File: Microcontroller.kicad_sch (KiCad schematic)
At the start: 31 parts, among them SW1 KMR221GLFS, U4 STM32F446RET6, U7 W25Q128JVSIQ, Y1 16MHz

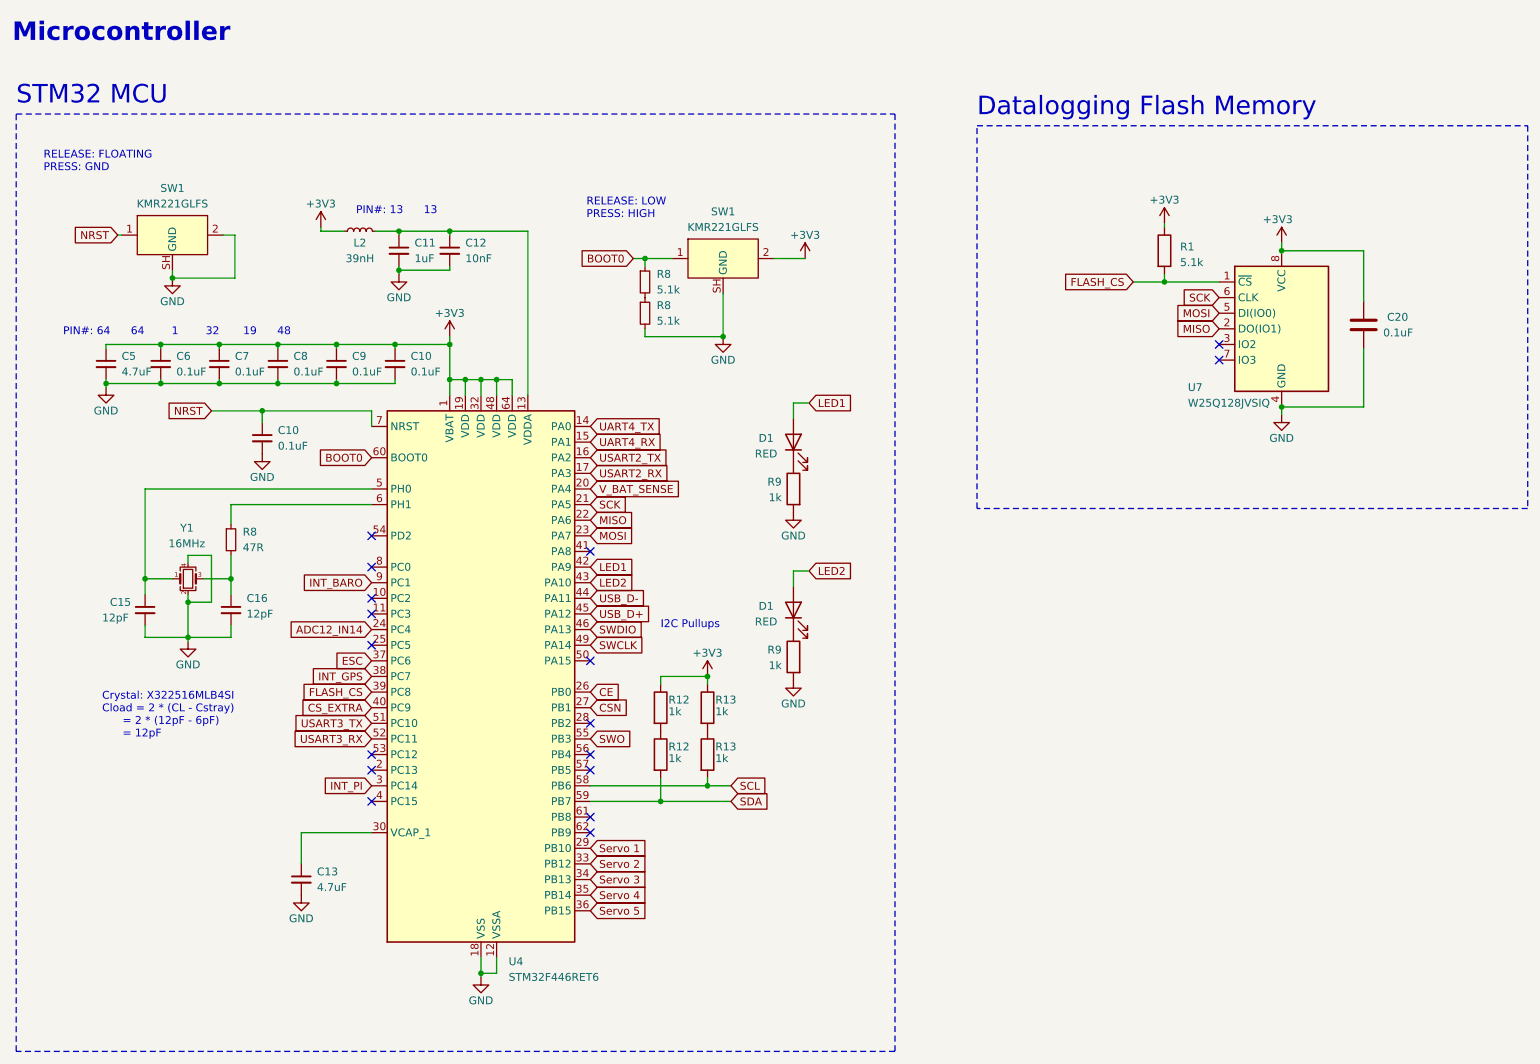
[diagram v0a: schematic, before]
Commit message: Add files via upload
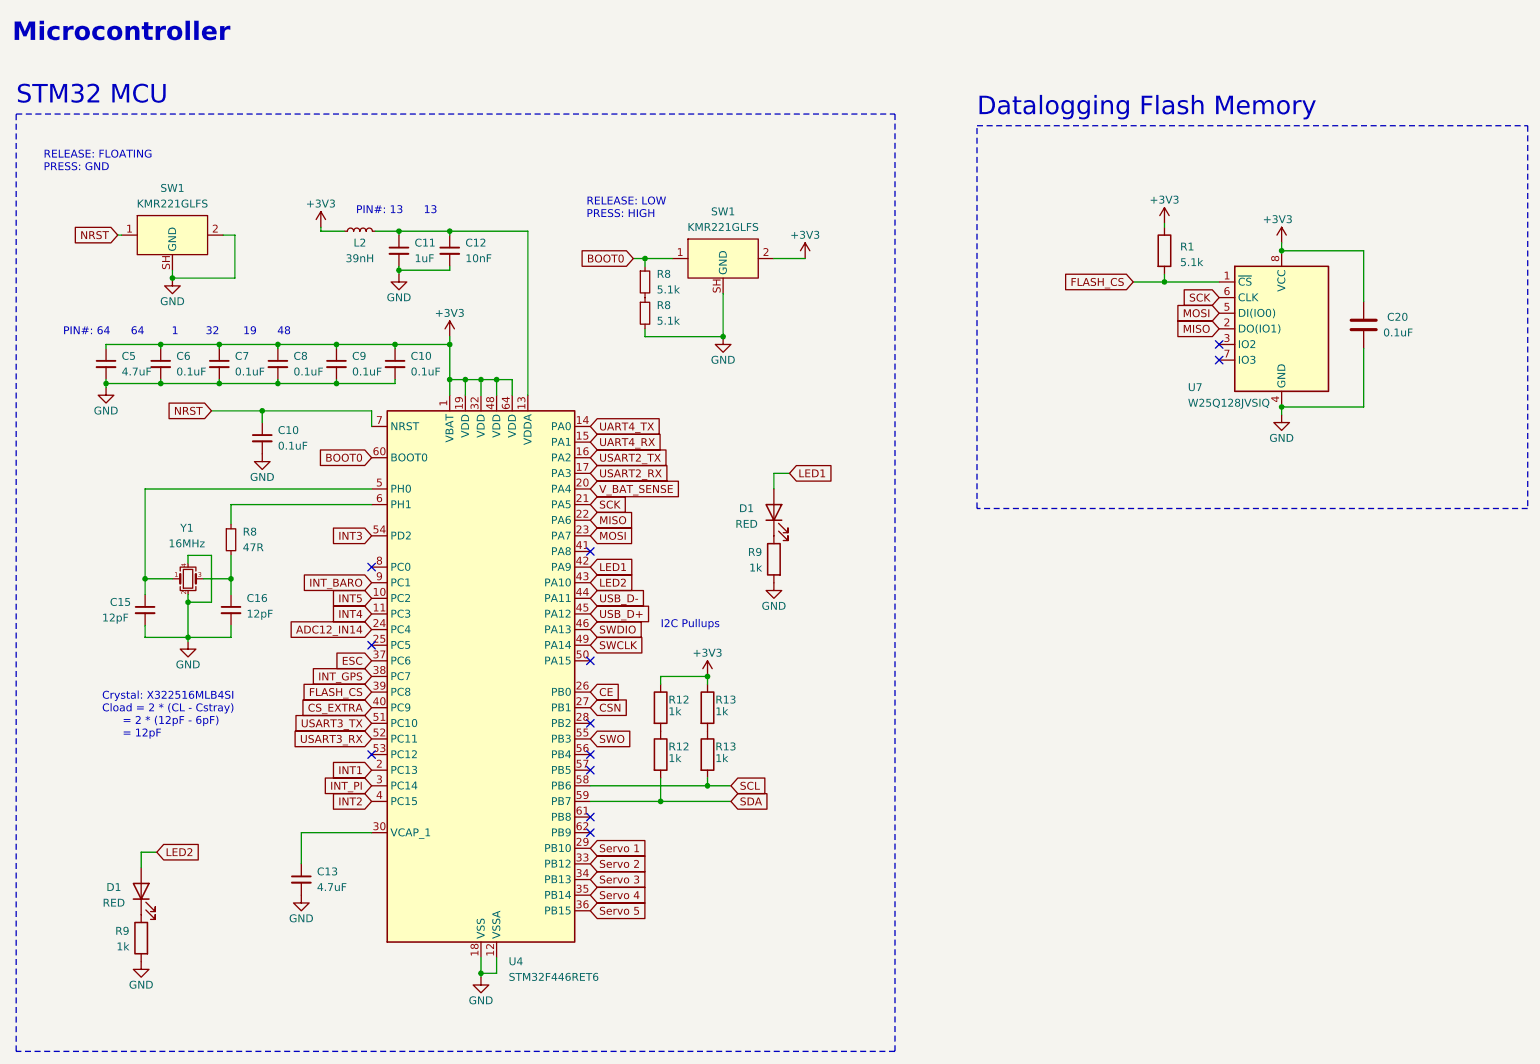
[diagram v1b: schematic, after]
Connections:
- net INT5: now reaches U4.10 (PC2)
- net INT4: now reaches U4.11 (PC3)
- net INT1: now reaches U4.2 (PC13)
- net INT2: now reaches U4.4 (PC15)
- net INT3: now reaches U4.54 (PD2)
- no-connect marks 17 -> 12
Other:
- moved on the sheet: D1, R9

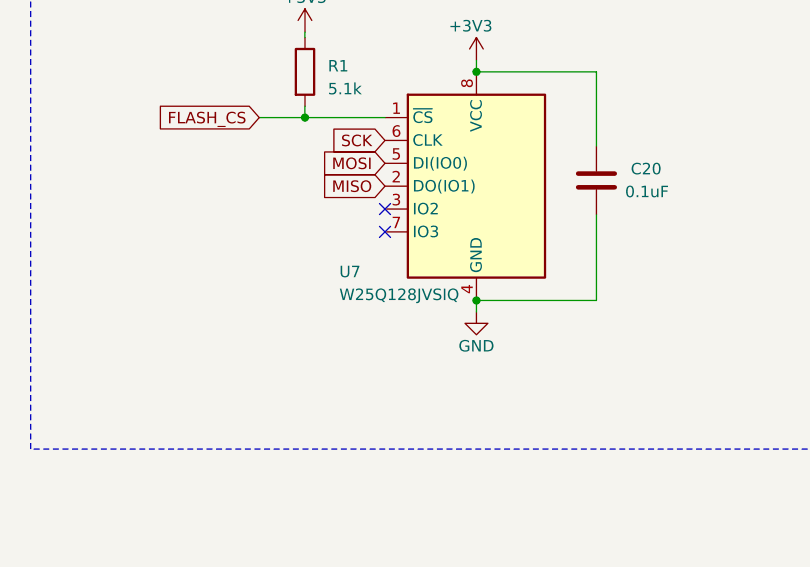
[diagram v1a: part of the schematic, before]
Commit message: Add files via upload
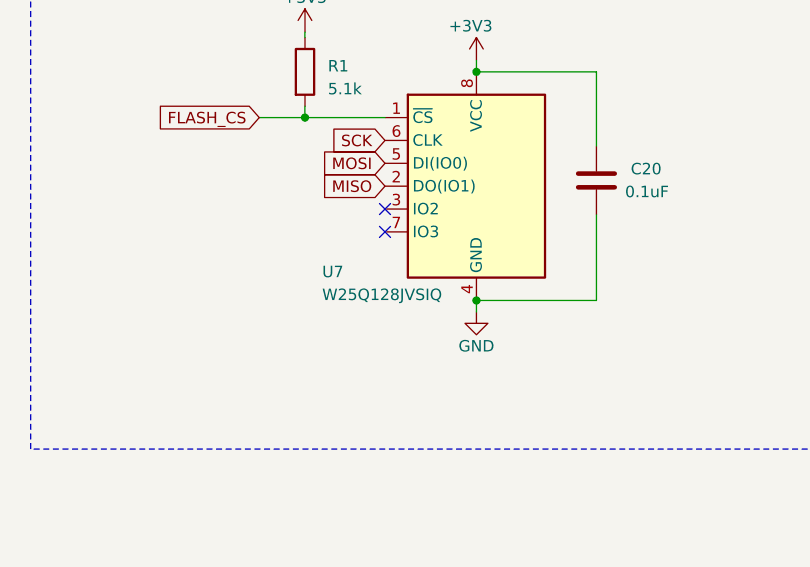
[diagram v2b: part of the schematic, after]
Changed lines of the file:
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@@
   (symbol (lib_id "Memory_Flash:W25Q128JVS") (at 229.87 69.85 0) (unit 1)
     (in_bom yes) (on_board yes) (dnp no)
-    (property "Reference" "U7" (at 214.63 79.375 0)
+    (property "Reference" "U7" (at 212.725 79.375 0)
       (effects (font (size 1.27 1.27)) (justify left))
     )
-    (property "Value" "W25Q128JVSIQ" (at 214.63 81.915 0)
+    (property "Value" "W25Q128JVSIQ" (at 212.725 81.915 0)
       (effects (font (size 1.27 1.27)) (justify left))
     )

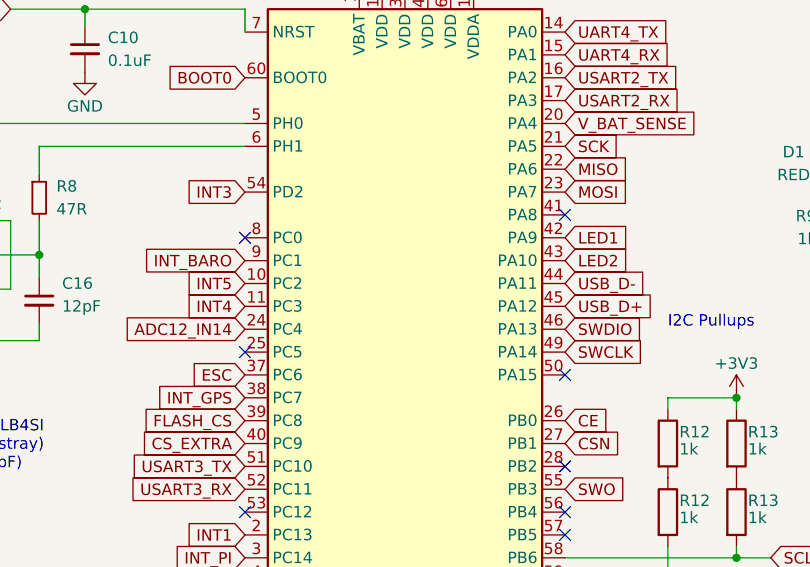
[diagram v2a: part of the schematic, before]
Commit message: Add files via upload
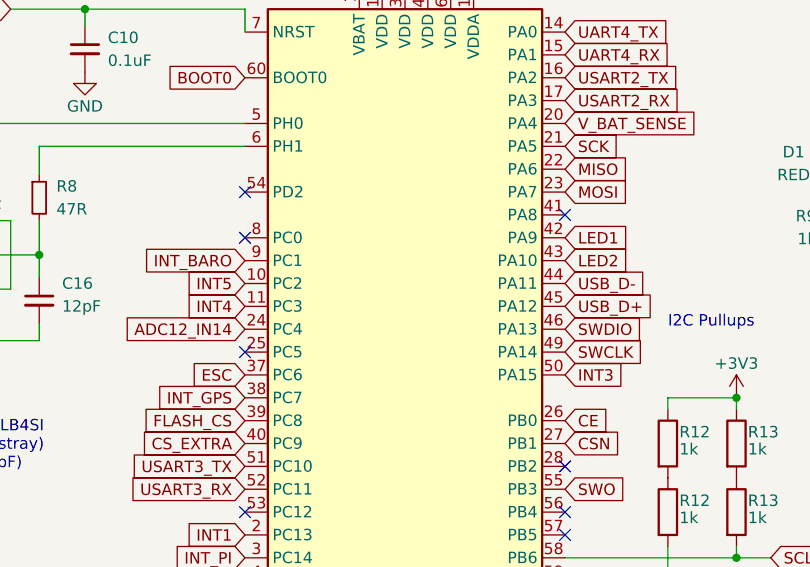
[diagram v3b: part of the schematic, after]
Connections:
- net INT3: now also U4.50 (PA15); no longer U4.54 (PD2)
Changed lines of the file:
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@@
   (no_connect (at 219.71 74.93))
   (no_connect (at 117.475 133.985))
-  (no_connect (at 117.475 123.825))
   (no_connect (at 117.475 149.225))
   (no_connect (at 81.915 108.585))
@@
   (no_connect (at 117.475 141.605))
   (no_connect (at 117.475 139.065))
+  (no_connect (at 81.915 103.505))
   (no_connect (at 117.475 151.765))
   (wire (pts (xy 46.99 154.94) (xy 44.45 154.94))
@@
     )
   )
-  (global_label "INT3" (shape input) (at 81.915 103.505 180) (fields_autoplaced)
-    (effects (font (size 1.27 1.27)) (justify right))
-    (property "Intersheetrefs" "${INTERSHEET_REFS}" (at 74.8968 103.505 0)
-      (effects (font (size 1.27 1.27)) (justify right) hide)
-    )
-  )
+  (global_label "INT3" (shape input) (at 117.475 123.825 0) (fields_autoplaced)
+    (effects (font (size 1.27 1.27)) (justify left))
+    (property "Intersheetrefs" "${INTERSHEET_REFS}" (at 124.4932 123.825 0)
+      (effects (font (size 1.27 1.27)) (justify left) hide)
+    )
+  )

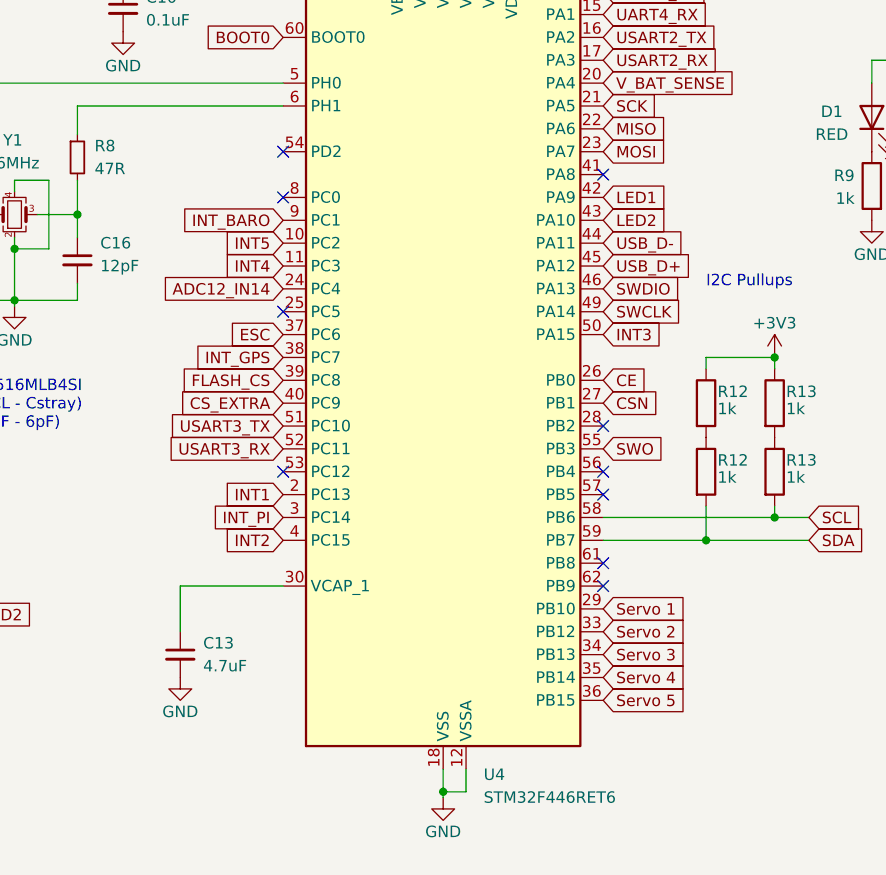
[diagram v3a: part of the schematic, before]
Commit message: Add files via upload
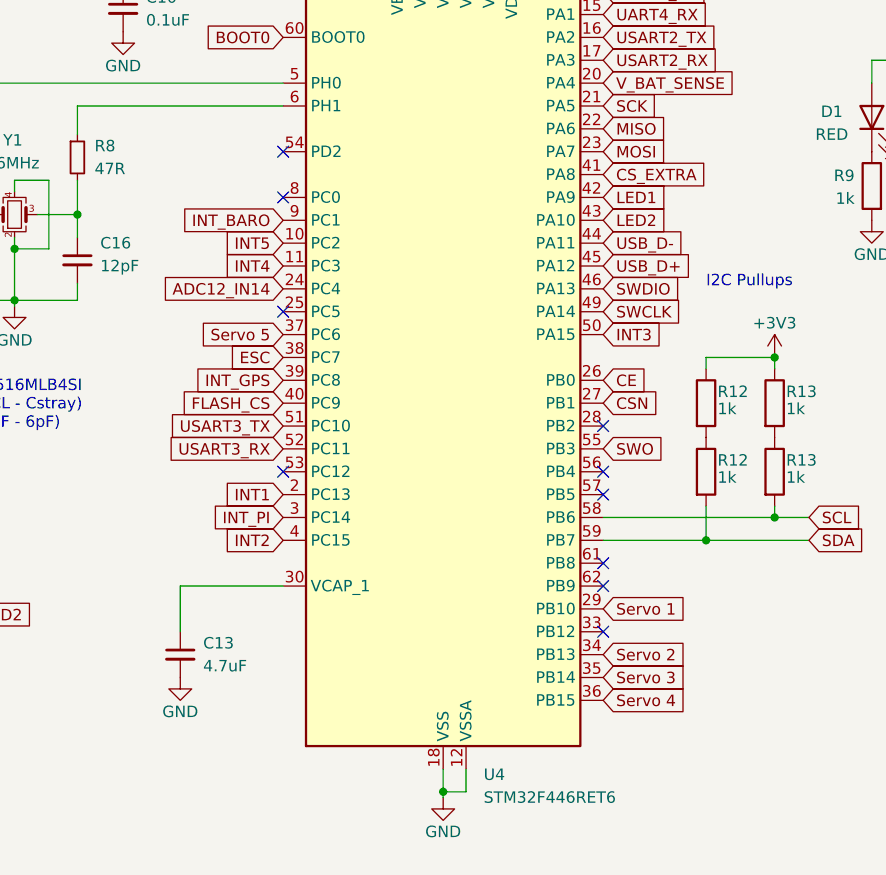
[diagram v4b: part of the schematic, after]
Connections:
- net CS_EXTRA: now also U4.41 (PA8); no longer U4.40 (PC9)
- net ESC: now also U4.38 (PC7); no longer U4.37 (PC6)
- net FLASH_CS: now also U4.40 (PC9); no longer U4.39 (PC8)
- net INT_GPS: now also U4.39 (PC8); no longer U4.38 (PC7)
- net Servo 2: now also U4.34 (PB13); no longer U4.33 (PB12)
- net Servo 3: now also U4.35 (PB14); no longer U4.34 (PB13)
- net Servo 4: now also U4.36 (PB15); no longer U4.35 (PB14)
- net Servo 5: now also U4.37 (PC6); no longer U4.36 (PB15)
